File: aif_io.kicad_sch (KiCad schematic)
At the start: 23 parts, among them J1 PWR, J3 CAN, J3 ST-LINK, J4 CAN, J5 AMT21, U1 THVD1420D

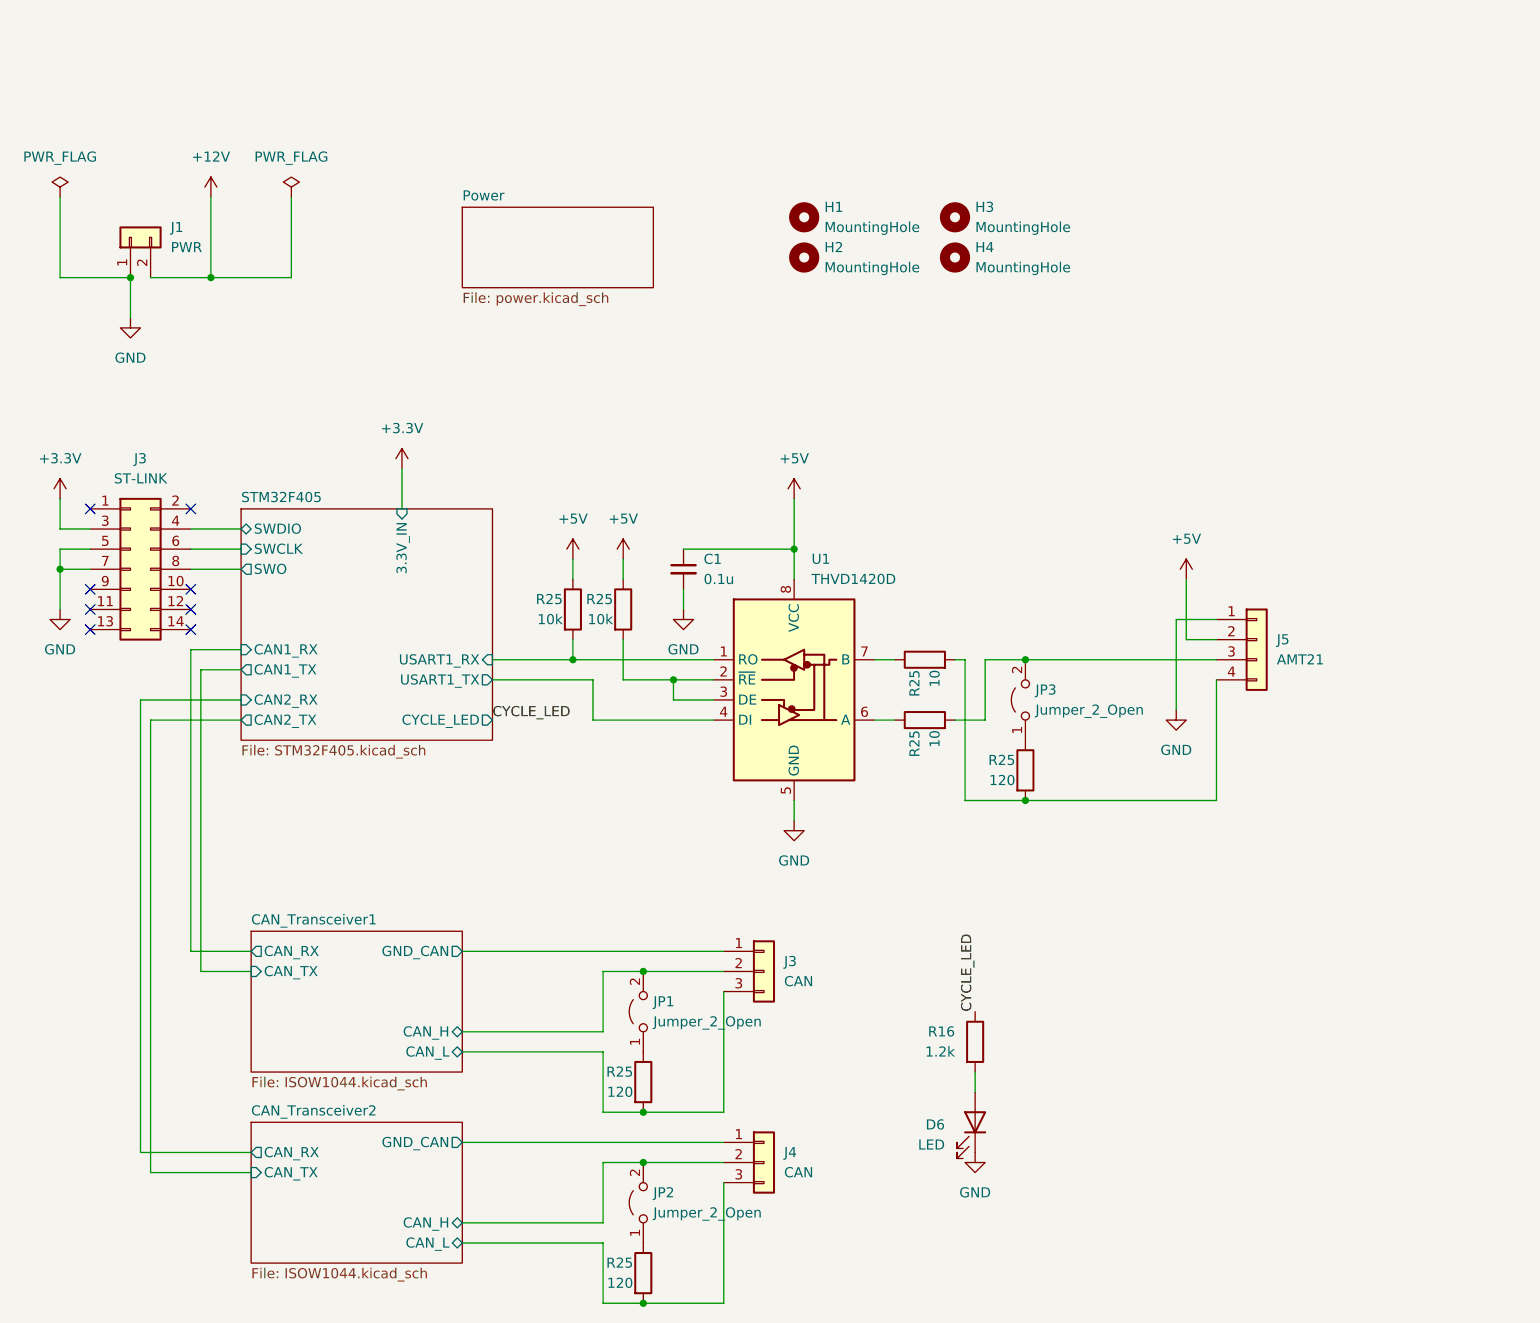
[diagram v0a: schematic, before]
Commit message: v0.2
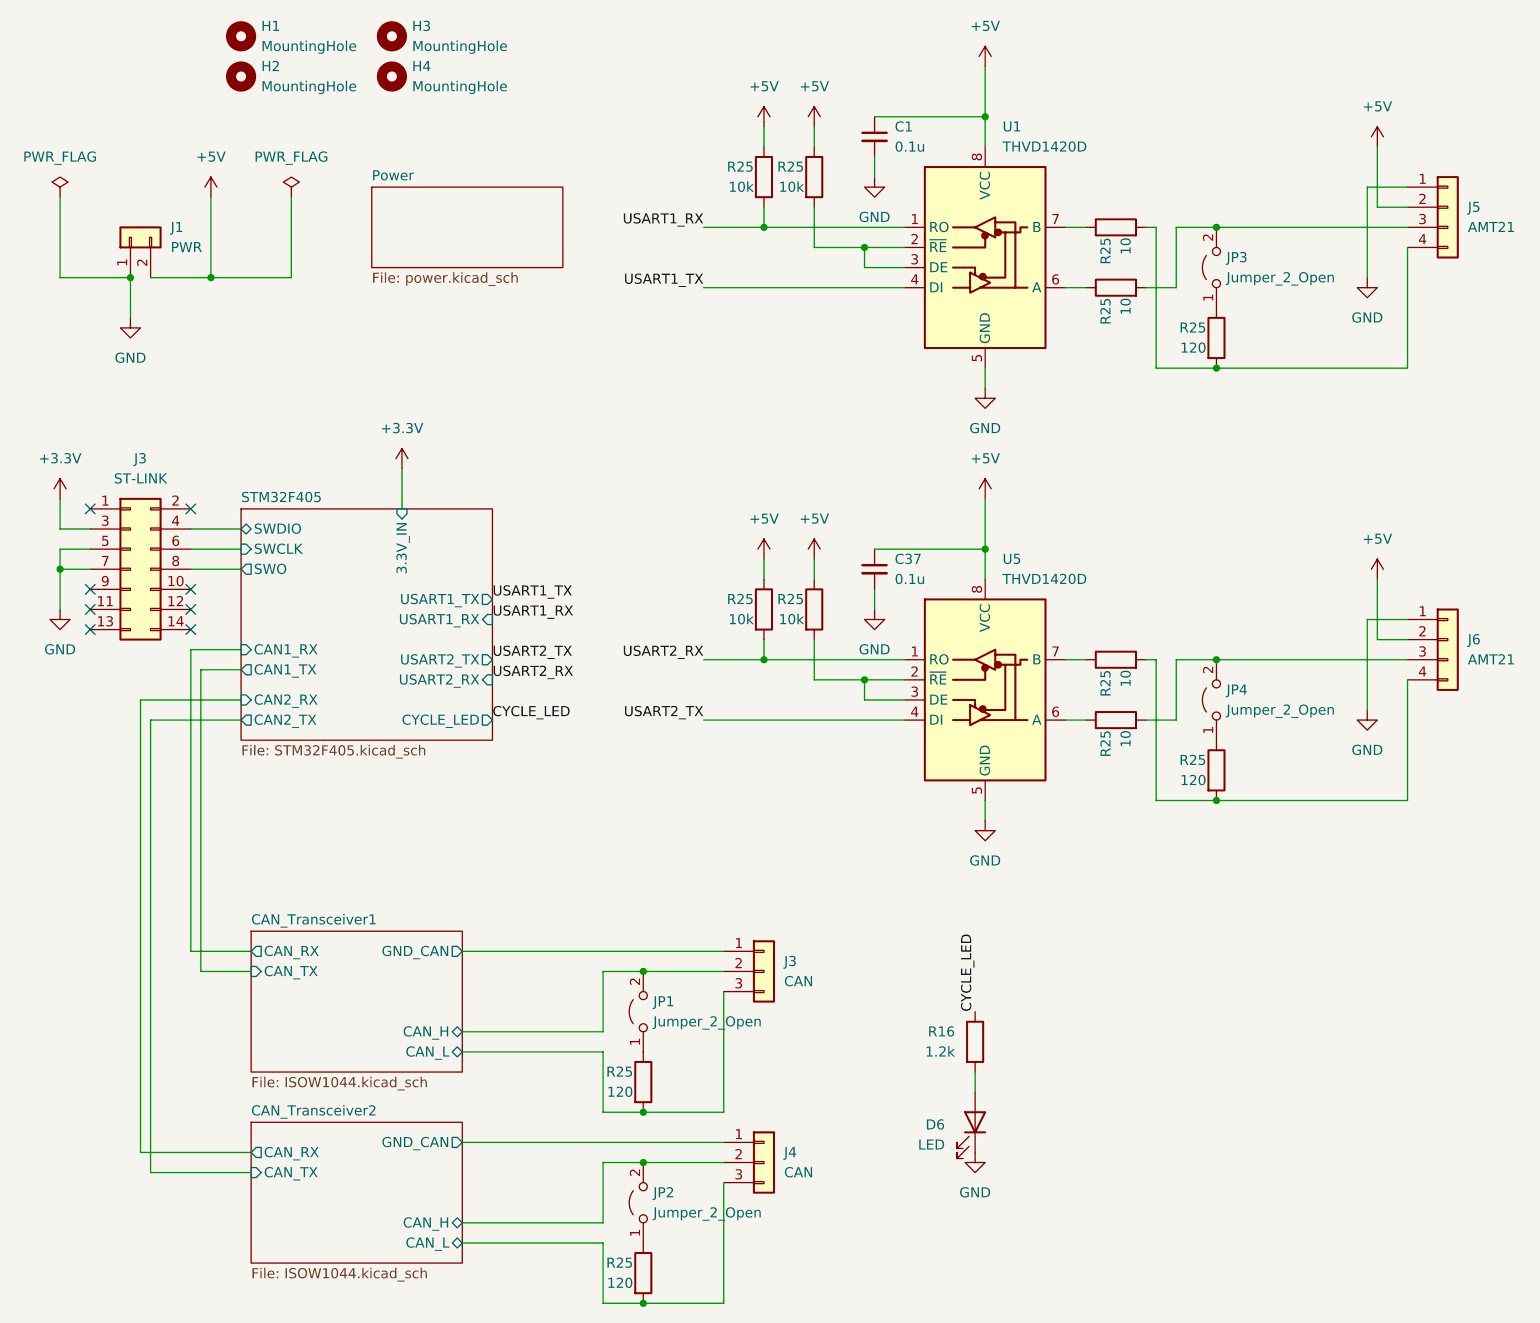
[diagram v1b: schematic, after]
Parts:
- added C37: 0.1u, Capacitor_SMD:C_0603_1608Metric, symbol Device:C_Small
- added J6: AMT21, Connector_JST:JST_XA_B04B-XASK-1_1x04_P2.50mm_Vertical, symbol Connector_Generic:Conn_01x04
- added JP4: Jumper_2_Open, Connector_PinHeader_2.54mm:PinHeader_1x02_P2.54mm_Vertical, symbol Jumper:Jumper_2_Open
- added R25 (x2): 10, Resistor_SMD:R_0603_1608Metric, symbol Device:R
- added R25: 120, Resistor_SMD:R_0603_1608Metric, symbol Device:R
- added R25 (x2): 10k, Resistor_SMD:R_0603_1608Metric, symbol Device:R
- added U5: THVD1420D, Package_SO:SOIC-8_3.9x4.9mm_P1.27mm, symbol Interface_UART:THVD1420D
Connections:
- net +12V is gone; now on net +5V: J1.2 (Pin_2)
- net +5V: now also C37.1, J6.2 (Pin_2), R25.1, R25.1, U5.8 (VCC)
- net GND: now also C37.2, J6.1 (Pin_1), U5.5 (GND)
- net STM32F405/USART1_RX renamed USART1_RX
- net STM32F405/USART1_TX renamed USART1_TX
- new net: R25.1, U5.7 (B)
- new net: J6.4 (Pin_4), R25.2, R25.2
- new net: J6.3 (Pin_3), JP4.2 (B), R25.2
- new net: JP4.1 (A), R25.1
- new net: R25.1, U5.6 (A)
- new net: R25.2, U5.2 (~{RE}), U5.3 (DE)
- new net USART2_RX: R25.2, U5.1 (RO)
- new net USART2_TX: U5.4 (DI)
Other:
- sheet STM32F405 ports: added USART2_RX, USART2_TX; removed none
- moved on the sheet: C1, H1, H2, H3, H4, J5, JP3, R25, U1
